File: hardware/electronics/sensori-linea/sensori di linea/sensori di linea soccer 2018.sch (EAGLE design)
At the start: 21 parts, among them T1 BP103, T2 BP103, T3 BP103, T4 BP103

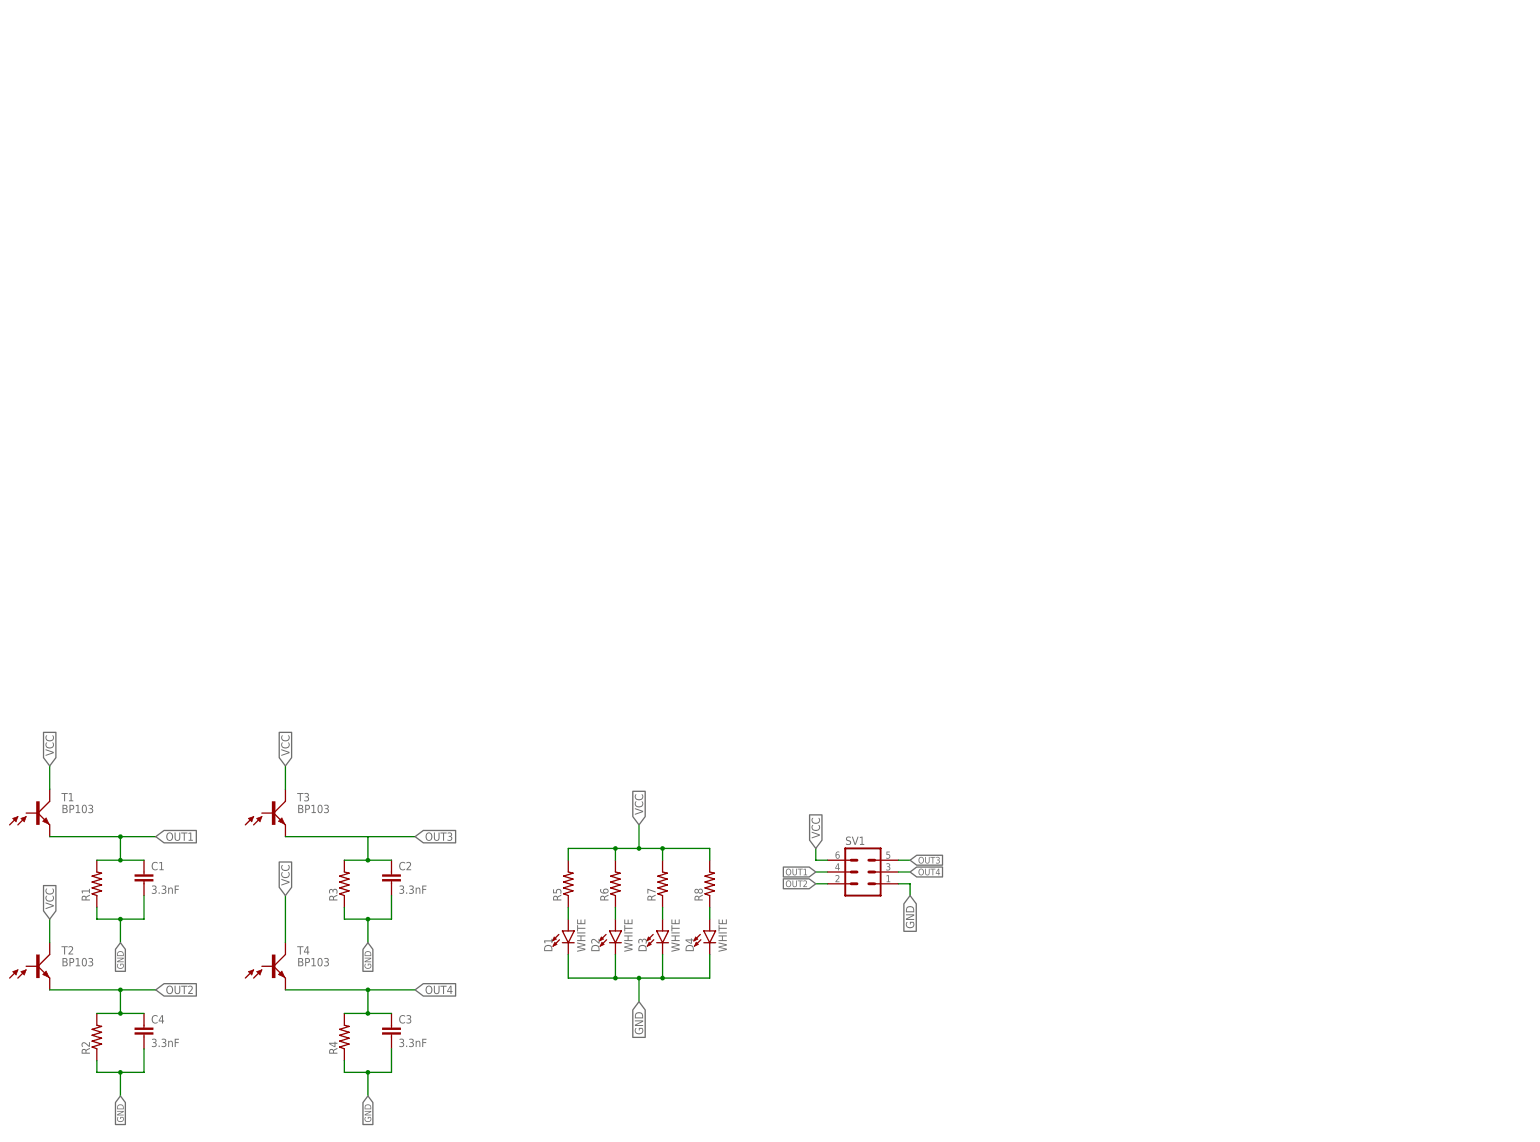
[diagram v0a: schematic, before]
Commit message: modfiche
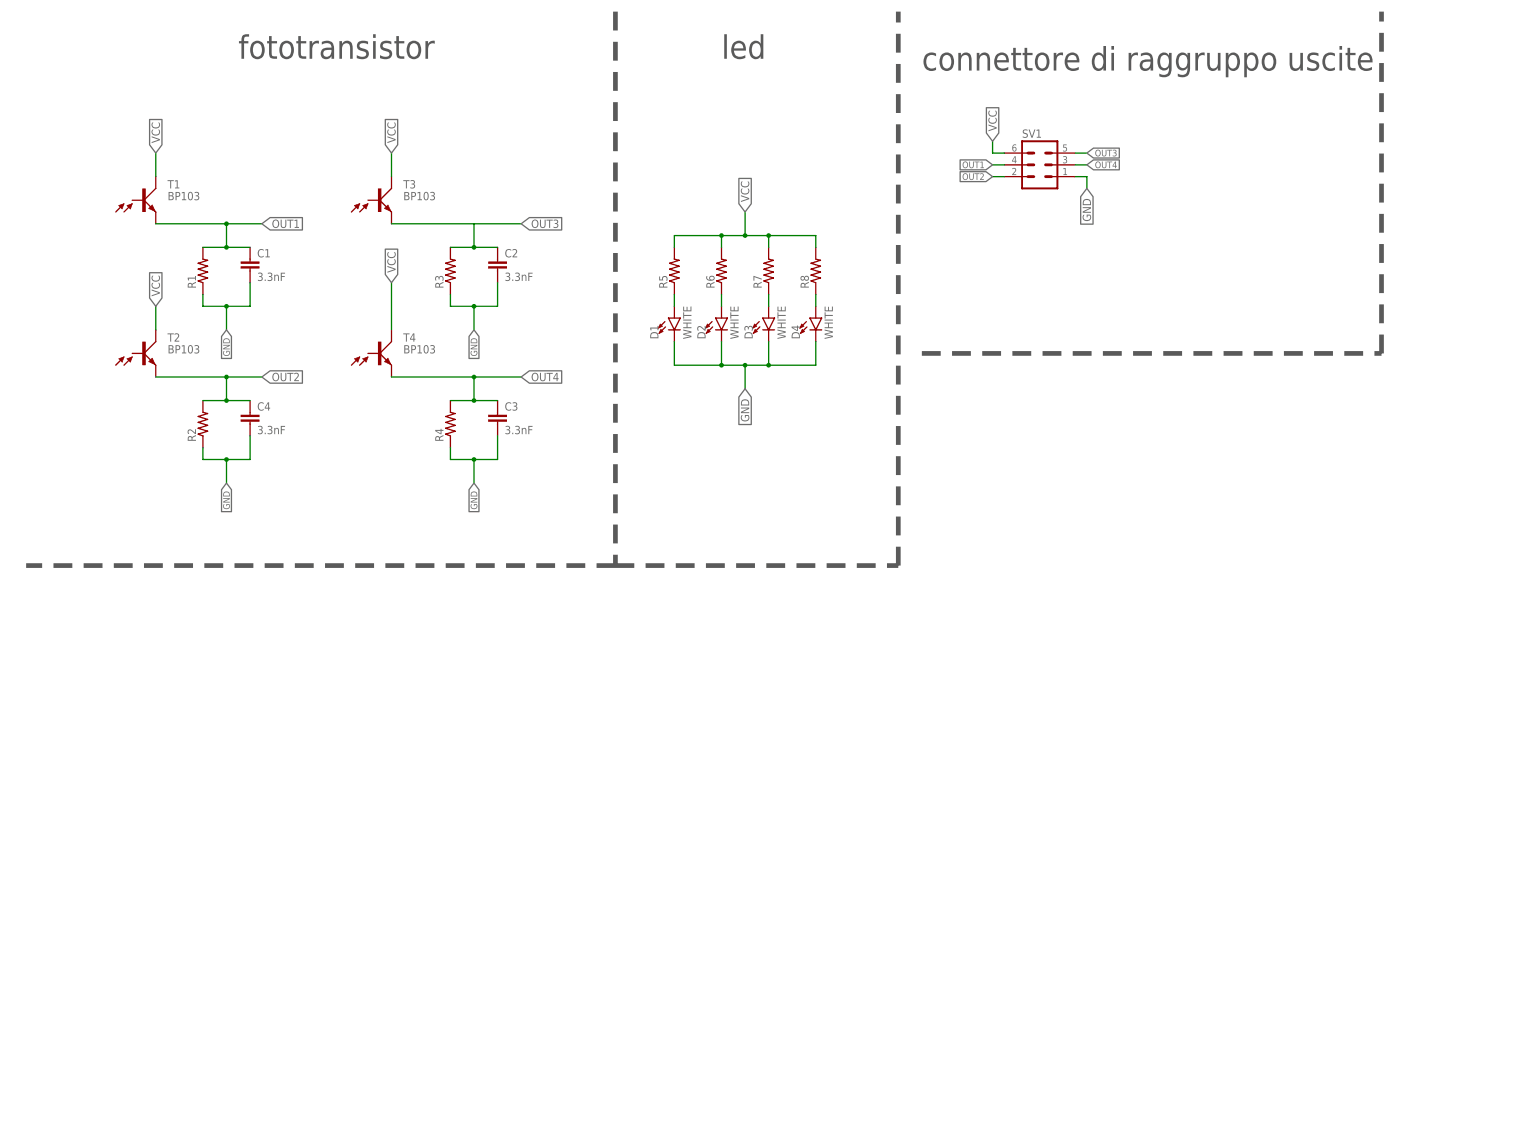
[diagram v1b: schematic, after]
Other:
- note added: "connettore di raggruppo uscite"
- note added: "fototransistor"
- note added: "led"
- moved on the sheet: C1, C2, C3, C4, D1, D2, D3, D4, R1, R2, R3, R4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
